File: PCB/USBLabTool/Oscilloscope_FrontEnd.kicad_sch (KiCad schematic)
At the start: 61 parts, among them J1 Chanel 1 input, J10 GPIO, J11 T_buf, J12 T_N5V, J13 ADC, J14 +3.3 V, J2 2174507-2, J3 T_att, J4 Conn_01x01, J5 T_acdc, J6 T_P5V, J7 T_amp, J8 T_pwm, J9 Conn_01x01, K1 G5V-2, Q1 IRLML6402TRPBF, U12 LMP7718, U2 AQY284SX, U3 CD74HC4316M96, U5 LTC1983ES6-5#TRPBF, U6 OPA863

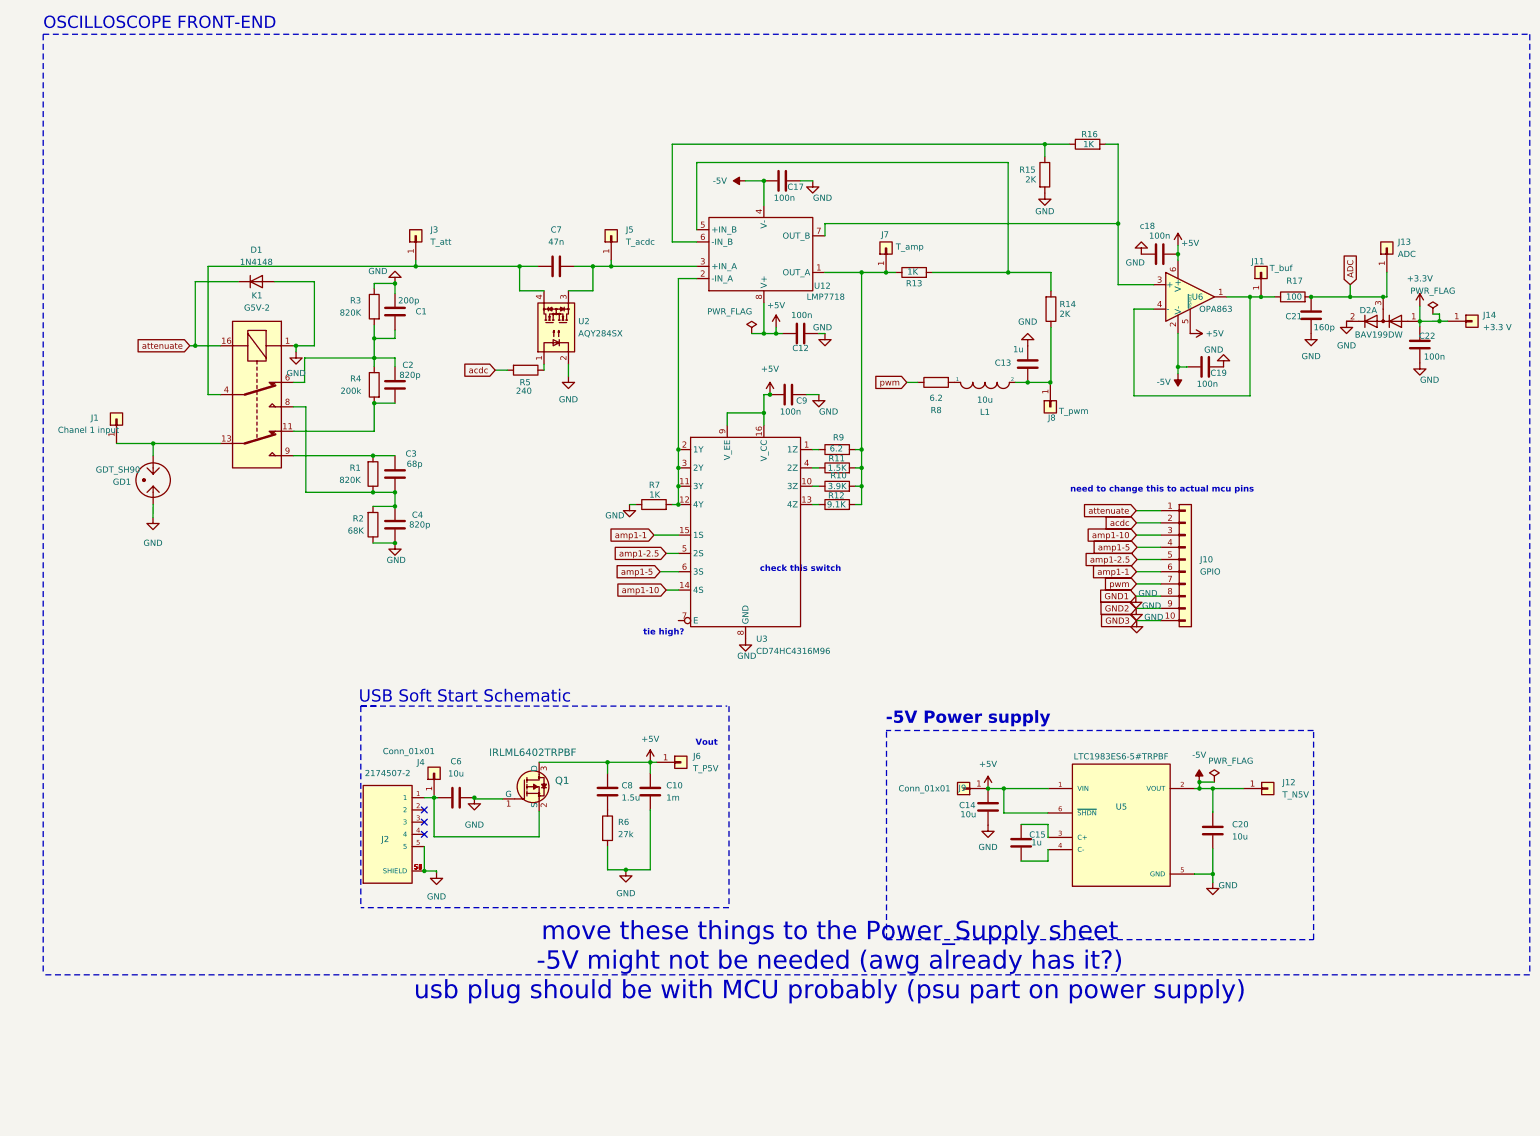
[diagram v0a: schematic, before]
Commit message: Starting PCB layout
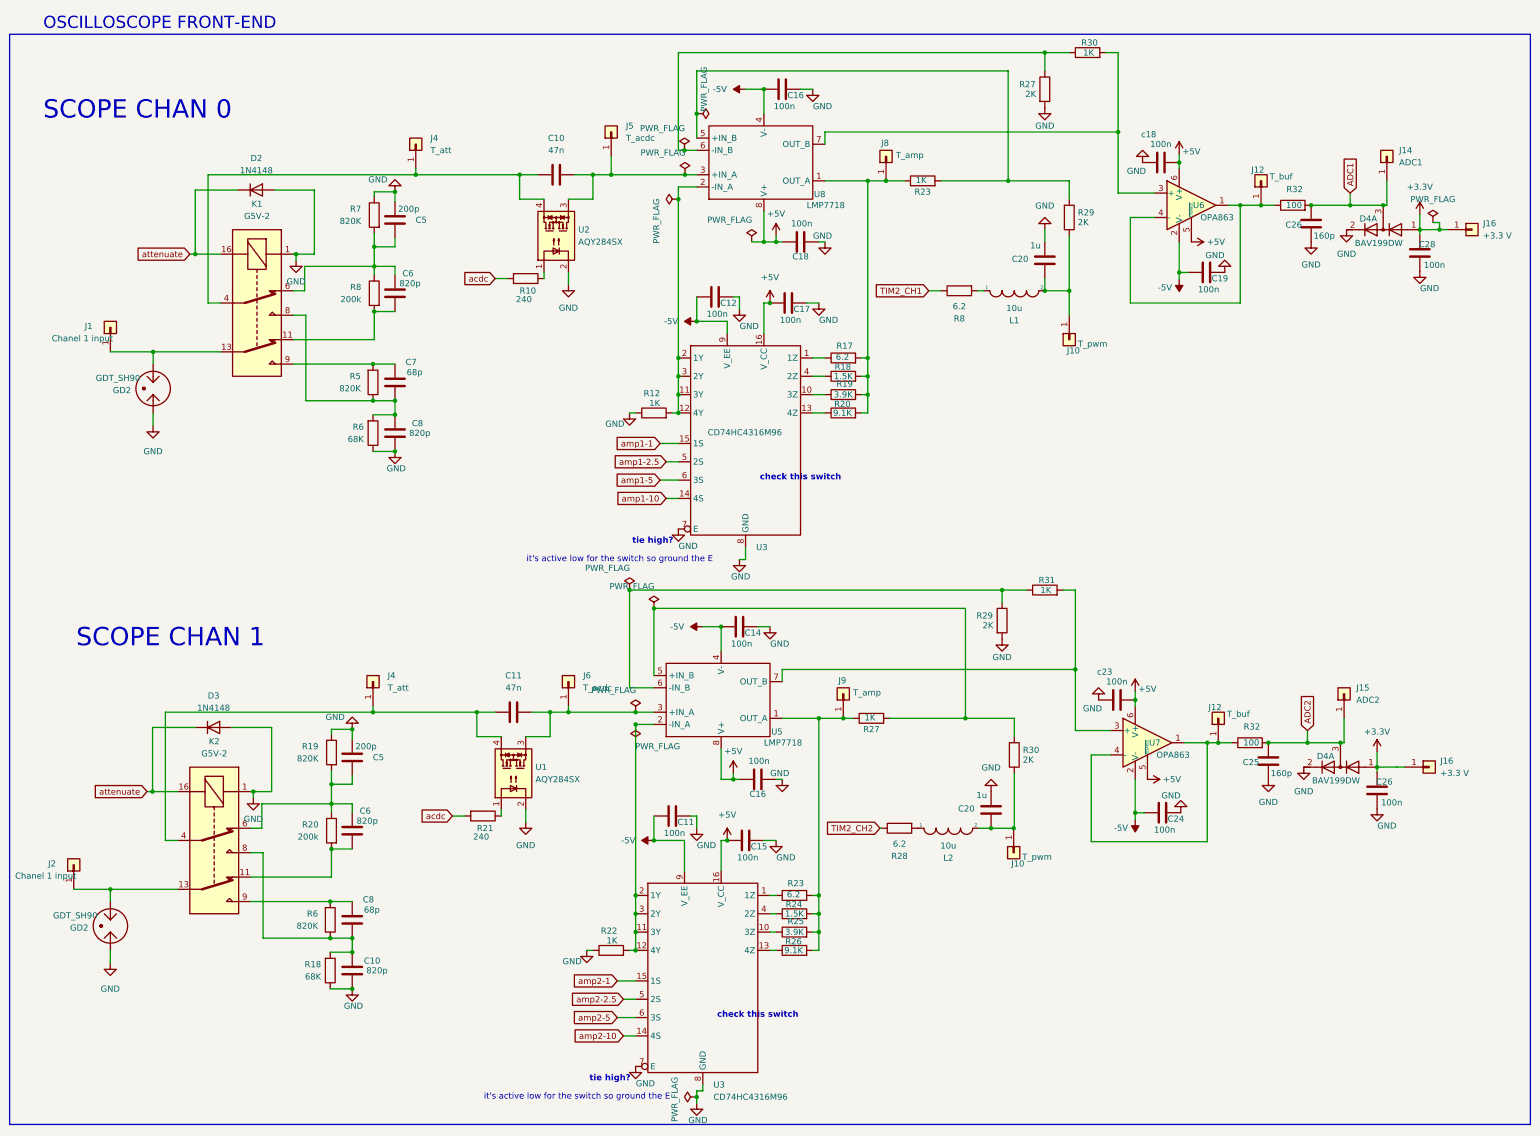
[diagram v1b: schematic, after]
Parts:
- removed J10: GPIO, Connector_PinHeader_2.54mm:PinHeader_1x10_P2.54mm_Vertical, symbol Connector_Generic:Conn_01x10
- removed J2: 2174507-2, J_SMD_2174507-2-5_7.8_5_2.71, symbol 2174507-2:2174507-2
- removed Q1: IRLML6402TRPBF, digikey-footprints:SOT-23-3, symbol dk_Transistors-FETs-MOSFETs-Single:IRLML6402TRPBF
- removed U12: LMP7718, Package_SO:VSSOP-8_3x3mm_P0.65mm, symbol USBLabTool:LMP7718MM/NOPB
- removed U3: CD74HC4316M96, symbol USBLabTool:CD74HC4316M96
- removed U5: LTC1983ES6-5#TRPBF, Package_TO_SOT_SMD:SOT-23-6_Handsoldering, symbol LTC1983ES6-5_TRPBF:LTC1983ES6-5#TRPBF
- added C11, C12, C16, C24, C26, c23: 100n, Capacitor_SMD:C_0603_1608Metric_Pad1.08x0.95mm_HandSolder, symbol Device:C
- added C11: 47n, Capacitor_SMD:C_0603_1608Metric_Pad1.08x0.95mm_HandSolder, symbol Device:C
- added C25: 160p, Capacitor_SMD:C_0603_1608Metric_Pad1.08x0.95mm_HandSolder, symbol Device:C
- added C5: 200p, Capacitor_SMD:C_0603_1608Metric_Pad1.08x0.95mm_HandSolder, symbol Device:C
- added D3: 1N4148, Diode_THT:D_DO-35_SOD27_P7.62mm_Horizontal, symbol Diode:1N4148
- added D4: BAV199DW, Package_TO_SOT_SMD:SOT-23, symbol Diode:BAV199DW
- added GD2: GDT_SH90, footprints:GDT_SH_LTF, symbol Device:GDT_2Pin
- added J10: T_pwm, Connector_PinHeader_2.54mm:PinHeader_1x01_P2.54mm_Vertical, symbol Connector_Generic:Conn_01x01
- added J15: ADC2, Connector_PinHeader_2.54mm:PinHeader_1x01_P2.54mm_Vertical, symbol Connector_Generic:Conn_01x01
- added J16: +3.3 V, Connector_PinHeader_2.54mm:PinHeader_1x01_P2.54mm_Vertical, symbol Connector_Generic:Conn_01x01
- added J2: Chanel 1 input, Connector_PinHeader_2.54mm:PinHeader_1x01_P2.54mm_Vertical, symbol Connector_Generic:Conn_01x01
- added K2: G5V-2, Relay_THT:Relay_DPDT_Omron_G5V-2, symbol Relay:G5V-2
- added L2: 10u, Inductor_SMD:L_0603_1608Metric_Pad1.05x0.95mm_HandSolder, symbol pspice:INDUCTOR
- added R18: 68K, Resistor_SMD:R_0603_1608Metric_Pad0.98x0.95mm_HandSolder, symbol Device:R
- added R19: 820K, Resistor_SMD:R_0603_1608Metric_Pad0.98x0.95mm_HandSolder, symbol Device:R
- added R20: 200k, Resistor_SMD:R_0603_1608Metric_Pad0.98x0.95mm_HandSolder, symbol Device:R
- added R21: 240, Resistor_SMD:R_0603_1608Metric_Pad0.98x0.95mm_HandSolder, symbol Device:R
- added R22, R27, R31: 1K, Resistor_SMD:R_0603_1608Metric_Pad0.98x0.95mm_HandSolder, symbol Device:R
- added R23, R28: 6.2, Resistor_SMD:R_0603_1608Metric_Pad0.98x0.95mm_HandSolder, symbol Device:R
- added R24: 1.5K, Resistor_SMD:R_0603_1608Metric_Pad0.98x0.95mm_HandSolder, symbol Device:R
- added R25: 3.9K, Resistor_SMD:R_0603_1608Metric_Pad0.98x0.95mm_HandSolder, symbol Device:R
- added R26: 9.1K, Resistor_SMD:R_0603_1608Metric_Pad0.98x0.95mm_HandSolder, symbol Device:R
- added R29, R30: 2K, Resistor_SMD:R_0603_1608Metric_Pad0.98x0.95mm_HandSolder, symbol Device:R
- added R32: 100, Resistor_SMD:R_0603_1608Metric_Pad0.98x0.95mm_HandSolder, symbol Device:R
- added U1: AQY284SX, Package_SO:SOP-4_3.8x4.1mm_P2.54mm, symbol Relay_SolidState:TLP3123
- added U3 (x2): CD74HC4316M96, Package_SO:SOIC-16_3.9x9.9mm_P1.27mm, symbol USBLabTool:CD74HC4316M96
- added U5, U8: LMP7718, Package_SO:VSSOP-8_3x3mm_P0.65mm, symbol USBLabTool:LMP7718MM/NOPB
- added U7: OPA863, Package_TO_SOT_SMD:SOT-23-6_Handsoldering, symbol Amplifier_Operational:ADA4807-1
- C10: value 1m -> 820p
- C14: value 10u -> 100n
- C15: value 1u -> 100n
- C20: value 10u -> 1u
- C6: value 10u -> 820p
- C8: value 1.5u -> 68p
- GD2: renamed from GD1; footprint digikey-footprints:SH90_1 -> footprints:GDT_SH_LTF
- J12: value T_N5V -> T_buf
- J14: renamed from J13; value ADC -> ADC1
- J4: value Conn_01x01 -> T_att
- J6: value T_P5V -> T_acdc
- J9: value Conn_01x01 -> T_amp
- R6: value 27k -> 820K
- renumbered C7 to C10, C17 to C16, C9 to C17, C12 to C18, C13 to C20, C21 to C26, C22 to C28, C1 to C5, C2 to C6, C3 to C7, C4 to C8, D1 to D2, D2 to D4, J8 to J10, J11 to J12, J14 to J16, J3 to J4, J7 to J8, R5 to R10, R7 to R12, R9 to R17, R11 to R18, R10 to R19, R12 to R20, R13 to R23, R15 to R27, R14 to R29, R16 to R30, R17 to R32, R1 to R5, R2 to R6, R3 to R7, R4 to R8
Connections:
- net +3.3V: now also C26.1, D4.1 (A1), J16.1 (Pin_1)
- net +5V: now also C15.1, C16.1, U3.16 (V_CC), U3.16 (V_CC), U5.8 (V+), U7.5 (~{DISABLE}), U7.6 (V+), U8.8 (V+), c23.2; no longer C10.1, C14.1, C8.2, J6.1 (Pin_1), J9.1 (Pin_1)
- net -5V: now also C14.1, C11.1, C12.1, C24.1, U3.9 (V_EE), U3.9 (V_EE), U5.4 (V-), U7.2 (V-), U8.4 (V-); no longer C20.1, J12.1 (Pin_1)
- net GND: now also C15.2, C11.2, C12.2, C16.2, C24.2, C25.2, C26.2, C5.1, D3.2 (A), D4.2 (K2), GD2.2, K2.1, R18.1, R19.1, R22.1, R29.2, U1.2, U3.7 (E), U3.7 (E), U3.8 (GND), U3.8 (GND), c23.1; no longer C6.2, R6.2
- net acdc: now also R21.2
- net amp1-1: now also U3.15 (1S)
- net amp1-10: now also U3.14 (4S)
- net amp1-2.5: now also U3.5 (2S)
- net amp1-5: now also U3.6 (3S)
- net attenuate: now also D3.1 (K), K2.16
- net at C10.2, J5.1 (Pin_1), U2.3: now also U8.3 (+IN_A)
- net at C6.1: now also C5.2, K2.6, R19.2, R20.1; no longer J4.1 (Pin_1)
- net at J8.1 (Pin_1), R17.2, R18.2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: now also U8.1 (OUT_A)
- net at R17.1: now also U3.1 (1Z)
- net at R27.1, R30.1: now also U8.6 (-IN_B)
- net at R20.1: now also U3.13 (4Z)
- net at R23.2, R29.2: now also U8.5 (+IN_B)
- net at R12.2: now also U3.11 (3Y), U3.12 (4Y), U3.2 (1Y), U3.3 (2Y), U8.2 (-IN_A)
- net at R30.2, U6.3 (+): now also U8.7 (OUT_B)
- net at R6.1: now also C10.1, C8.2, K2.8, R18.2; no longer C8.1
- net at R19.1: now also U3.10 (3Z)
- net at R18.1: now also U3.4 (2Z)
- net ADC renamed ADC1
- net pwm renamed TIM2_CH1
- new net: C8.1, K2.9, R6.2
- new net: R23.1, U3.1 (1Z)
- new net: J9.1 (Pin_1), R23.2, R24.2, R25.2, R26.2, R27.1, U5.1 (OUT_A)
- new net: R25.1, U3.10 (3Z)
- new net: R29.1, R31.1, U5.6 (-IN_B)
- new net: R31.2, U5.7 (OUT_B), U7.3 (+)
- new net: J12.1 (Pin_1), R32.1, U7.1, U7.4 (-)
- new net: C20.1, J10.1 (Pin_1), L2.2, R30.1
- new net: R27.2, R30.2, U5.5 (+IN_B)
- new net: R24.1, U3.4 (2Z)
- new net: R22.2, U3.11 (3Y), U3.12 (4Y), U3.2 (1Y), U3.3 (2Y), U5.2 (-IN_A)
- new net: C6.2, K2.11, R20.2
- new net: C11.2, J6.1 (Pin_1), U1.3, U5.3 (+IN_A)
- new net: R21.1, U1.1
- new net: C11.1, J4.1 (Pin_1), K2.4, U1.4
- new net: GD2.1, J2.1 (Pin_1), K2.13
- new net: R26.1, U3.13 (4Z)
- new net: L2.1, R28.2
- new net ADC2: C25.1, D4.3 (K3A4), J15.1 (Pin_1), R32.2
- new net TIM2_CH2: R28.1
- new net amp2-1: U3.15 (1S)
- new net amp2-10: U3.14 (4S)
- new net amp2-2.5: U3.5 (2S)
- new net amp2-5: U3.6 (3S)
- no-connect marks 3 -> 0
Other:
- note added: "SCOPE CHAN 0"
- note added: "SCOPE CHAN 1"
- note added: "it's active low for the switch so ground the E"
- note removed: "-5V Power supply"
- note removed: "USB Soft Start Schematic"
- note removed: "Vout"
- note removed: "move these things to the Power_Supply sheet -5V might not be needed (awg already has it?) usb plug should be with MCU probably (psu part on power supply)"
- note removed: "need to change this to actual mcu pins"
- moved on the sheet: C10, C16, C17, C18, C20, C26, C28, C5, C6, C7, C8, D2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
